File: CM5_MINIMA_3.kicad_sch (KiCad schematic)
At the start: 22 parts, among them J101 TYPEC-305-ACP16H458, SW101 MK-11C04-G013

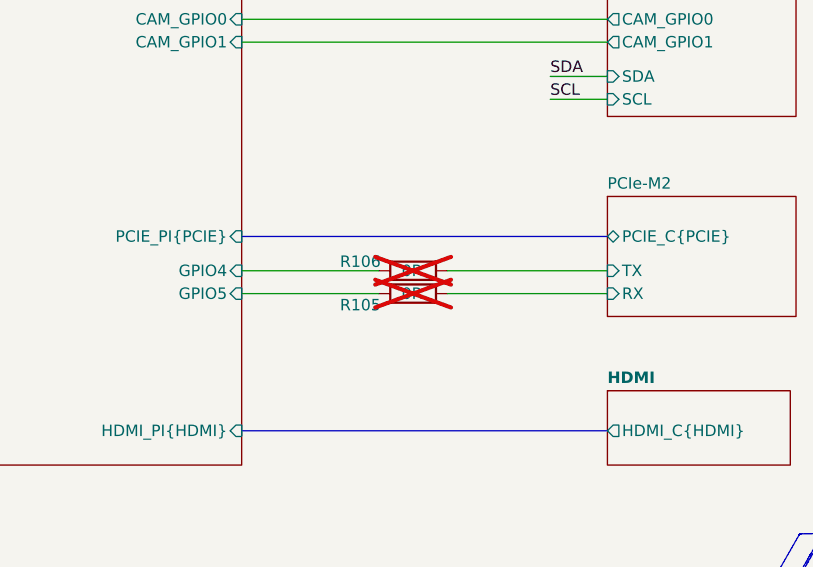
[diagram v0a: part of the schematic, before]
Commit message: DRC and prod files
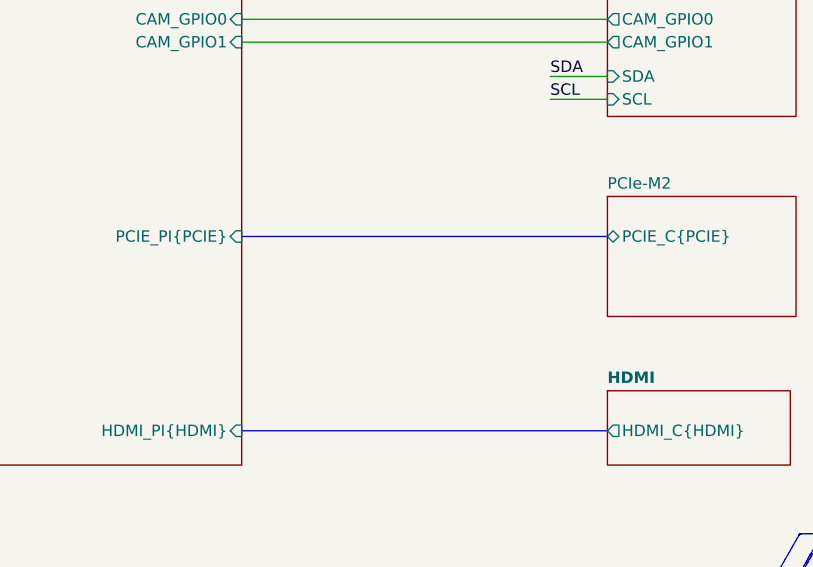
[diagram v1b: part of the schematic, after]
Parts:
- removed R105, R106: 0R, Resistor_SMD:R_0402_1005Metric, symbol Device:R
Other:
- sheet CM5 ports: added none; removed GPIO4, GPIO5
- sheet PCIe-M2 ports: added none; removed RX, TX
